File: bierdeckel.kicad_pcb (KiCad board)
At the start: 2 copper layers, 93 x 93 mm, 91 parts, among them IC1 HSFPAR004A, J1 Pogo, J2 Pogo, J3 Pogo, J4 Pogo, Q1 BSS138P,215, SW1 PTS526 SK15 SMTR2 LFS, SW2 PTS526 SK15 SMTR2 LFS, SW3 PTS526 SK15 SMTR2 LFS, U1 ESP32-C3-WROOM-02, U2 BQ25176J, U3 TPS61201DRC, U4 BQ51050BRHL, U6 INA317IDGKR

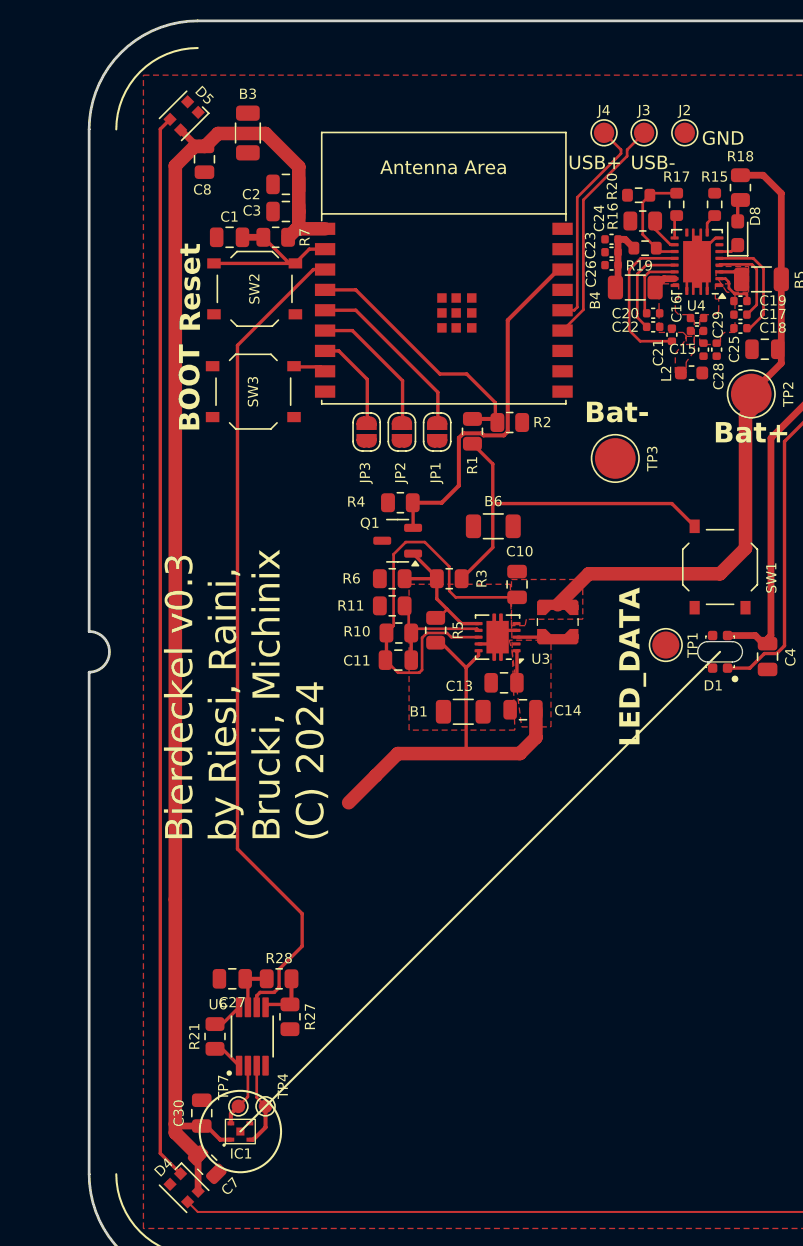
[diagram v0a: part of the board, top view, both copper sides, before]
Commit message: continue refactor
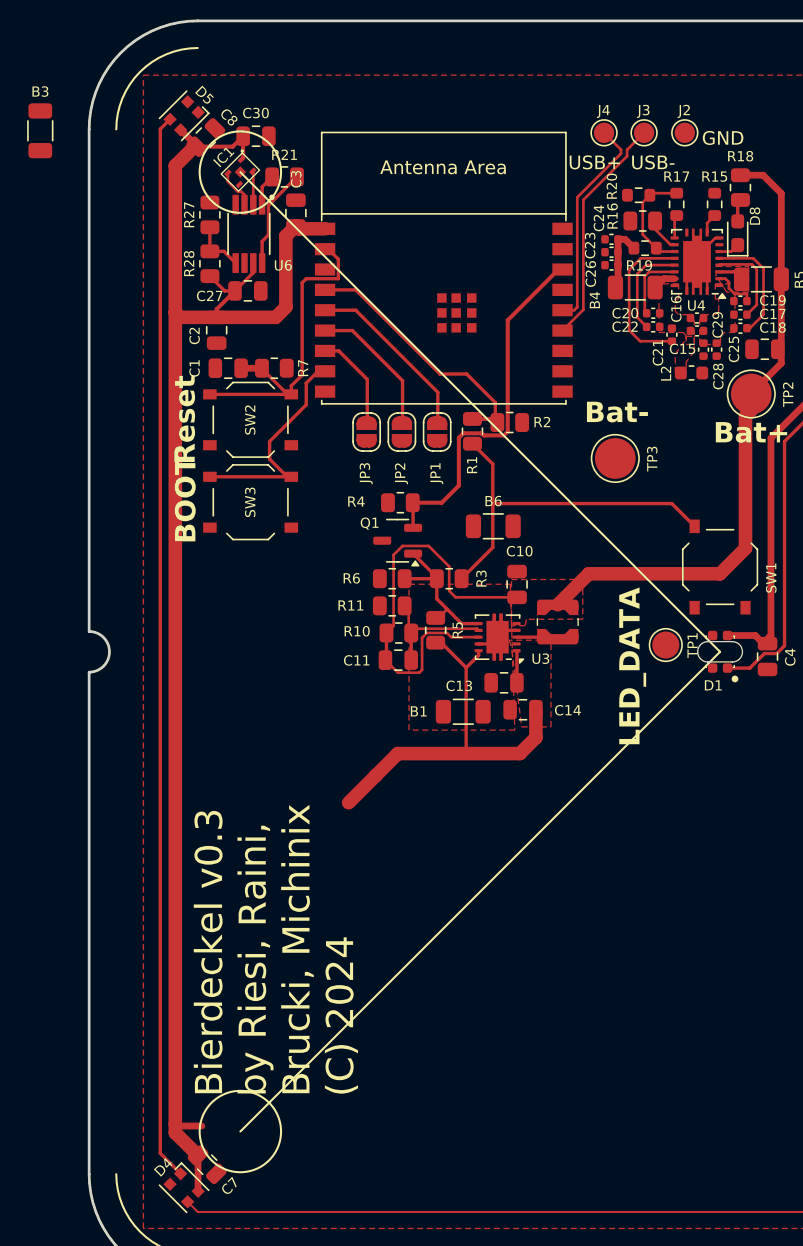
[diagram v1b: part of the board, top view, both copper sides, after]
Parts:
- removed TP4, TP7: TestPoint, TestPoint:TestPoint_Pad_D1.0mm
- moved C30 72.1 mm to (112.3, 58.5), turned to 0 degrees
- moved IC1 70.7 mm to (111.1, 61.1), turned to -45 degrees
- moved R21 63.6 mm to (114.4, 61.5), turned to 180 degrees
- moved R27 59.4 mm to (108.9, 64.3), turned to 90 degrees
- moved U6 59.2 mm to (111.8, 65.7), turned to -90 degrees
- moved R28 52.9 mm to (108.9, 67.9), turned to -90 degrees
- moved C27 50.7 mm to (111.7, 69.9), turned to 0 degrees
- moved B3 15.3 mm to (96.4, 58.1)
- moved C2 11.9 mm to (109.4, 72.8), turned to -90 degrees
- moved SW2 9.65 mm to (111.9, 79.4)
- moved C1 9.65 mm to (110.2, 75.6)
- moved R7 9.65 mm to (113.7, 75.6)
- moved SW3 8.15 mm to (111.9, 85.5)
- moved C8 1.60 mm to (108.6, 58.6), turned to 45 degrees
- moved C3 0.75 mm to (115.2, 64.2), turned to 90 degrees
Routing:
- net /Vpress: track 61.5 -> 0.00 mm
- net /~{BOOTLOADER}: track 2.45 -> 16.6 mm
- net /RST: track 13.4 -> 24.6 mm
- net +3.3V: track 295.3 -> 302.2 mm
- net Net-(U6-RG__1): track 2.29 -> 7.41 mm
- net /Pressure Gauge/VR+: track 6.35 -> 3.00 mm
- net /Pressure Gauge/VR-: track 4.78 -> 2.49 mm
